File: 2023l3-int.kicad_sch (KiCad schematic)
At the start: 9 parts, among them J1 0526101433, J2 52610-0833, SW1 SW_DIP_x04

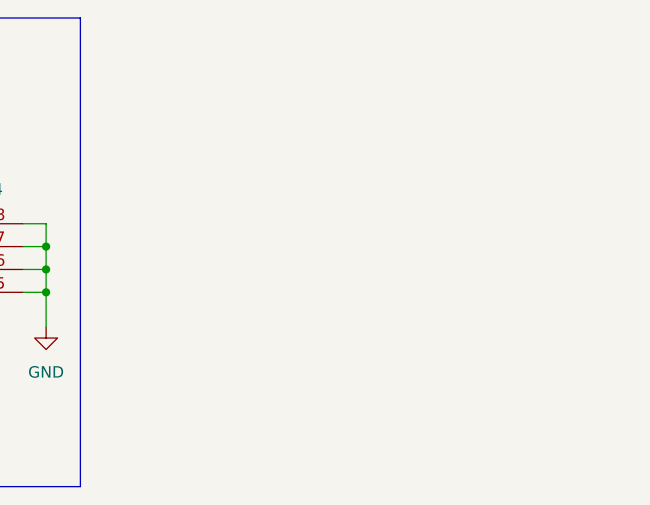
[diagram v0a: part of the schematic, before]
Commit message: kill me
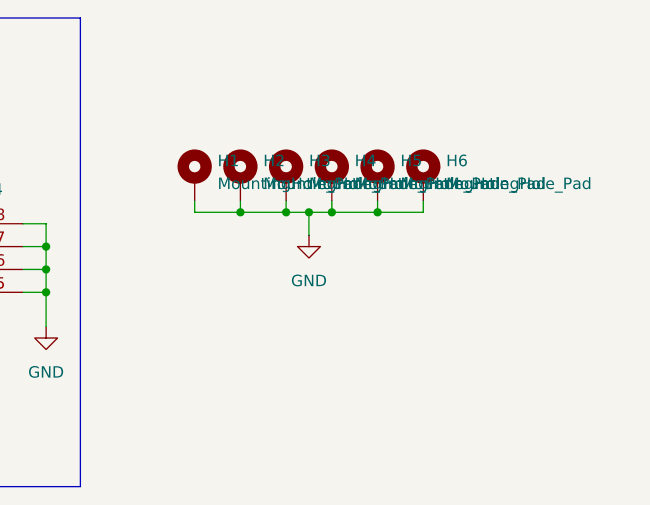
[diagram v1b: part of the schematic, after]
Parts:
- added H1, H2, H3, H4, H5, H6: MountingHole_Pad, MountingHole:MountingHole_3.2mm_M3_Pad_Via, symbol Mechanical:MountingHole_Pad
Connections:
- net GND: now also H1.1, H2.1, H3.1, H4.1, H5.1, H6.1
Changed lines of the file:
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@@
   (junction (at 88.9 45.72) (diameter 0) (color 0 0 0 0)
   )
+  (junction (at 232.41 36.83) (diameter 0) (color 0 0 0 0)
+  )
   (junction (at 205.74 43.18) (diameter 0) (color 0 0 0 0)
   )
+  (junction (at 242.57 36.83) (diameter 0) (color 0 0 0 0)
+  )
+  (junction (at 237.49 36.83) (diameter 0) (color 0 0 0 0)
+  )
   (junction (at 205.74 45.72) (diameter 0) (color 0 0 0 0)
+  )
+  (junction (at 227.33 36.83) (diameter 0) (color 0 0 0 0)
+  )
+  (junction (at 234.95 36.83) (diameter 0) (color 0 0 0 0)
   )
   (junction (at 205.74 40.64) (diameter 0) (color 0 0 0 0)
@@
   (no_connect (at 130.81 93.98))
   (no_connect (at 161.29 91.44))
+  (wire (pts (xy 222.25 35.56) (xy 222.25 36.83))
+    (stroke (width 0) (type default))
+  )
   (wire (pts (xy 123.19 36.83) (xy 132.08 36.83))
     (stroke (width 0) (type default))
@@
     (stroke (width 0) (type default))
   )
+  (wire (pts (xy 232.41 35.56) (xy 232.41 36.83))
+    (stroke (width 0) (type default))
+  )
   (wire (pts (xy 165.1 57.15) (xy 173.99 57.15))
     (stroke (width 0) (type default))
@@
     (stroke (width 0) (type default))
   )
+  (wire (pts (xy 227.33 36.83) (xy 232.41 36.83))
+    (stroke (width 0) (type default))
+  )
   (wire (pts (xy 35.56 87.63) (xy 35.56 88.9))
     (stroke (width 0) (type default))
@@
     (stroke (width 0) (type default))
   )
+  (wire (pts (xy 227.33 35.56) (xy 227.33 36.83))
+    (stroke (width 0) (type default))
+  )
   (wire (pts (xy 88.9 43.18) (xy 88.9 45.72))
     (stroke (width 0) (type default))
   )
+  (wire (pts (xy 232.41 36.83) (xy 234.95 36.83))
+    (stroke (width 0) (type default))
+  )
   (wire (pts (xy 124.46 101.6) (xy 130.81 101.6))
     (stroke (width 0) (type default))
@@
     (stroke (width 0) (type default))
   )
+  (wire (pts (xy 237.49 35.56) (xy 237.49 36.83))
+    (stroke (width 0) (type default))
+  )
   (wire (pts (xy 88.9 46.99) (xy 88.9 45.72))
     (stroke (width 0) (type default))
@@
     (stroke (width 0) (type default))
   )
+  (wire (pts (xy 222.25 36.83) (xy 227.33 36.83))
+    (stroke (width 0) (type default))
+  )
   (wire (pts (xy 165.1 39.37) (xy 175.26 39.37))
     (stroke (width 0) (type default))
@@
     (stroke (width 0) (type default))
   )
+  (wire (pts (xy 234.95 36.83) (xy 237.49 36.83))
+    (stroke (width 0) (type default))
+  )
   (wire (pts (xy 203.2 43.18) (xy 205.74 43.18))
     (stroke (width 0) (type default))
@@
     (stroke (width 0) (type default))
   )
+  (wire (pts (xy 237.49 36.83) (xy 242.57 36.83))
+    (stroke (width 0) (type default))
+  )
   (wire (pts (xy 205.74 43.18) (xy 205.74 45.72))
     (stroke (width 0) (type default))
@@
     (stroke (width 0) (type default))
   )
+  (wire (pts (xy 247.65 36.83) (xy 247.65 35.56))
+    (stroke (width 0) (type default))
+  )
   (wire (pts (xy 132.08 26.67) (xy 124.46 26.67))
     (stroke (width 0) (type default))
@@
   )
   (wire (pts (xy 123.19 49.53) (xy 132.08 49.53))
+    (stroke (width 0) (type default))
+  )
+  (wire (pts (xy 242.57 35.56) (xy 242.57 36.83))
+    (stroke (width 0) (type default))
+  )
+  (wire (pts (xy 242.57 36.83) (xy 247.65 36.83))
+    (stroke (width 0) (type default))
+  )
+  (wire (pts (xy 234.95 36.83) (xy 234.95 39.37))
     (stroke (width 0) (type default))
   )
@@
   (label "SCL" (at 125.73 99.06 0) (fields_autoplaced)
     (effects (font (size 1.27 1.27)) (justify left bottom))
+  )
+  (symbol (lib_id "Mechanical:MountingHole_Pad") (at 242.57 33.02 0) (unit 1)
+    (in_bom yes) (on_board yes) (dnp no) (fields_autoplaced)
+    (property "Reference" "H5" (at 245.11 31.115 0)
+      (effects (font (size 1.27 1.27)) (justify left))
+    )
+    (property "Value" "MountingHole_Pad" (at 245.11 33.655 0)
+      (effects (font (size 1.27 1.27)) (justify left))
+    )
+    (property "Footprint" "MountingHole:MountingHole_3.2mm_M3_Pad_Via" (at 242.57 33.02 0)
+      (effects (font (size 1.27 1.27)) hide)
+    )
+    (property "Datasheet" "~" (at 242.57 33.02 0)
+      (effects (font (size 1.27 1.27)) hide)
+    )
+    (pin "1")
+    (instances
+      (project "2023l3-int"
+        (path "/91e7b1c2-b009-4d84-9159-ee8884a12474"
+          (reference "H5") (unit 1)
+        )
+      )
+    )
   )
   (symbol (lib_id "Device:R_Photo") (at 35.56 83.82 0) (unit 1)
@@
     )
   )
+  (symbol (lib_id "Mechanical:MountingHole_Pad") (at 222.25 33.02 0) (unit 1)
+    (in_bom yes) (on_board yes) (dnp no) (fields_autoplaced)
+    (property "Reference" "H1" (at 224.79 31.115 0)
+      (effects (font (size 1.27 1.27)) (justify left))
+    )
+    (property "Value" "MountingHole_Pad" (at 224.79 33.655 0)
+      (effects (font (size 1.27 1.27)) (justify left))
+    )
+    (property "Footprint" "MountingHole:MountingHole_3.2mm_M3_Pad_Via" (at 222.25 33.02 0)
+      (effects (font (size 1.27 1.27)) hide)
+    )
+    (property "Datasheet" "~" (at 222.25 33.02 0)
+      (effects (font (size 1.27 1.27)) hide)
+    )
+    (pin "1")
+    (instances
+      (project "2023l3-int"
+        (path "/91e7b1c2-b009-4d84-9159-ee8884a12474"
+          (reference "H1") (unit 1)
+        )
+      )
+    )
+  )
+  (symbol (lib_id "Mechanical:MountingHole_Pad") (at 237.49 33.02 0) (unit 1)
+    (in_bom yes) (on_board yes) (dnp no) (fields_autoplaced)
+    (property "Reference" "H4" (at 240.03 31.115 0)
+      (effects (font (size 1.27 1.27)) (justify left))
+    )
+    (property "Value" "MountingHole_Pad" (at 240.03 33.655 0)
+      (effects (font (size 1.27 1.27)) (justify left))
+    )
+    (property "Footprint" "MountingHole:MountingHole_3.2mm_M3_Pad_Via" (at 237.49 33.02 0)
+      (effects (font (size 1.27 1.27)) hide)
+    )
+    (property "Datasheet" "~" (at 237.49 33.02 0)
+      (effects (font (size 1.27 1.27)) hide)
+    )
+    (pin "1")
+    (instances
+      (project "2023l3-int"
+        (path "/91e7b1c2-b009-4d84-9159-ee8884a12474"
+          (reference "H4") (unit 1)
+        )
+      )
+    )
+  )
   (symbol (lib_id "power:+5V") (at 88.9 35.56 270) (unit 1)
     (in_bom yes) (on_board yes) (dnp no) (fields_autoplaced)
@@
     )
   )
+  (symbol (lib_id "power:GND") (at 234.95 39.37 0) (unit 1)
+    (in_bom yes) (on_board yes) (dnp no) (fields_autoplaced)
+    (property "Reference" "#PWR011" (at 234.95 45.72 0)
+      (effects (font (size 1.27 1.27)) hide)
+    )
+    (property "Value" "GND" (at 234.95 44.45 0)
+      (effects (font (size 1.27 1.27)))
+    )
+    (property "Footprint" "" (at 234.95 39.37 0)
+      (effects (font (size 1.27 1.27)) hide)
+    )
+    (property "Datasheet" "" (at 234.95 39.37 0)
+      (effects (font (size 1.27 1.27)) hide)
+    )
+    (pin "1")
+    (instances
+      (project "2023l3-int"
+        (path "/91e7b1c2-b009-4d84-9159-ee8884a12474"
+          (reference "#PWR011") (unit 1)
+        )
+      )
+    )
+  )
   (symbol (lib_id "power:GND") (at 88.9 46.99 0) (unit 1)
     (in_bom yes) (on_board yes) (dnp no) (fields_autoplaced)
@@
         (path "/91e7b1c2-b009-4d84-9159-ee8884a12474"
           (reference "#PWR02") (unit 1)
+        )
+      )
+    )
+  )
+  (symbol (lib_id "Mechanical:MountingHole_Pad") (at 247.65 33.02 0) (unit 1)
+    (in_bom yes) (on_board yes) (dnp no) (fields_autoplaced)
+    (property "Reference" "H6" (at 250.19 31.115 0)
+      (effects (font (size 1.27 1.27)) (justify left))
+    )
+    (property "Value" "MountingHole_Pad" (at 250.19 33.655 0)
+      (effects (font (size 1.27 1.27)) (justify left))
+    )
+    (property "Footprint" "MountingHole:MountingHole_3.2mm_M3_Pad_Via" (at 247.65 33.02 0)
+      (effects (font (size 1.27 1.27)) hide)
+    )
+    (property "Datasheet" "~" (at 247.65 33.02 0)
+      (effects (font (size 1.27 1.27)) hide)
+    )
+    (pin "1")
+    (instances
+      (project "2023l3-int"
+        (path "/91e7b1c2-b009-4d84-9159-ee8884a12474"
+          (reference "H6") (unit 1)
         )
       )
@@
         (path "/91e7b1c2-b009-4d84-9159-ee8884a12474"
           (reference "D1") (unit 1)
+        )
+      )
+    )
+  )
+  (symbol (lib_id "Mechanical:MountingHole_Pad") (at 227.33 33.02 0) (unit 1)
+    (in_bom yes) (on_board yes) (dnp no) (fields_autoplaced)
+    (property "Reference" "H2" (at 229.87 31.115 0)
+      (effects (font (size 1.27 1.27)) (justify left))
+    )
+    (property "Value" "MountingHole_Pad" (at 229.87 33.655 0)
+      (effects (font (size 1.27 1.27)) (justify left))
+    )
+    (property "Footprint" "MountingHole:MountingHole_3.2mm_M3_Pad_Via" (at 227.33 33.02 0)
+      (effects (font (size 1.27 1.27)) hide)
+    )
+    (property "Datasheet" "~" (at 227.33 33.02 0)
+      (effects (font (size 1.27 1.27)) hide)
+    )
+    (pin "1")
+    (instances
+      (project "2023l3-int"
+        (path "/91e7b1c2-b009-4d84-9159-ee8884a12474"
+          (reference "H2") (unit 1)
         )
       )
@@
         )
       )
+    )
+  )
+  (symbol (lib_id "Mechanical:MountingHole_Pad") (at 232.41 33.02 0) (unit 1)
+    (in_bom yes) (on_board yes) (dnp no) (fields_autoplaced)
+    (property "Reference" "H3" (at 234.95 31.115 0)
+      (effects (font (size 1.27 1.27)) (justify left))
+    )
+    (property "Value" "MountingHole_Pad" (at 234.95 33.655 0)
+      (effects (font (size 1.27 1.27)) (justify left))
+    )
+    (property "Footprint" "MountingHole:MountingHole_3.2mm_M3_Pad_Via" (at 232.41 33.02 0)
+      (effects (font (size 1.27 1.27)) hide)
+    )
+    (property "Datasheet" "~" (at 232.41 33.02 0)
+      (effects (font (size 1.27 1.27)) hide)
+    )
+    (pin "1")
+    (instances
+      (project "2023l3-int"
+        (path "/91e7b1c2-b009-4d84-9159-ee8884a12474"
+          (reference "H3") (unit 1)
+        )
+      )
